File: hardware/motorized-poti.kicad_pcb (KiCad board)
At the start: 2 copper layers, 100 x 18 mm, 18 parts, among them J1 AKL_5_2, P1 CON-SENSOR, P2 MOTORIZED_POTI, U1 M24C64, U2 ZXBM5210, U3 DRILL, U4 DRILL, U5 DRILL, U6 DRILL

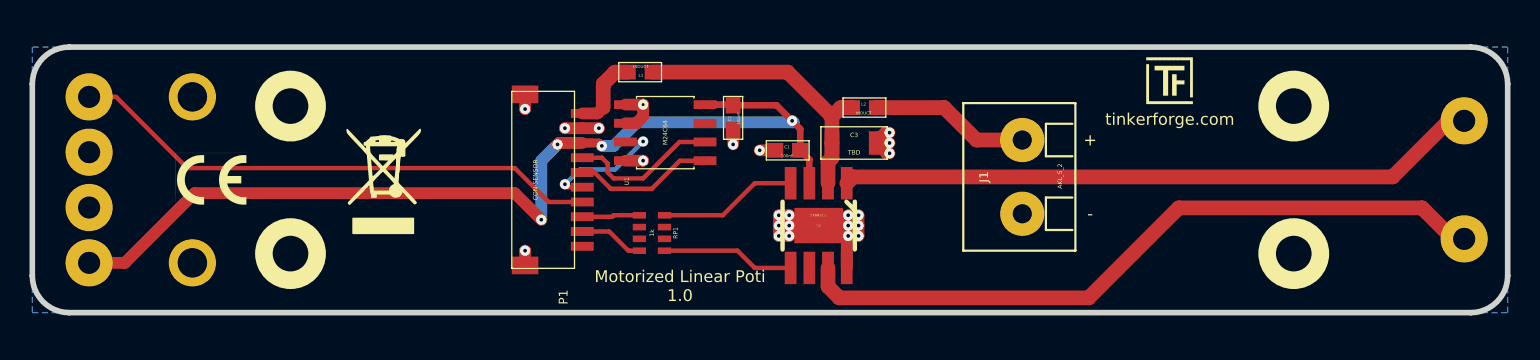
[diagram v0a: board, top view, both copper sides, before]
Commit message: restore proto placement
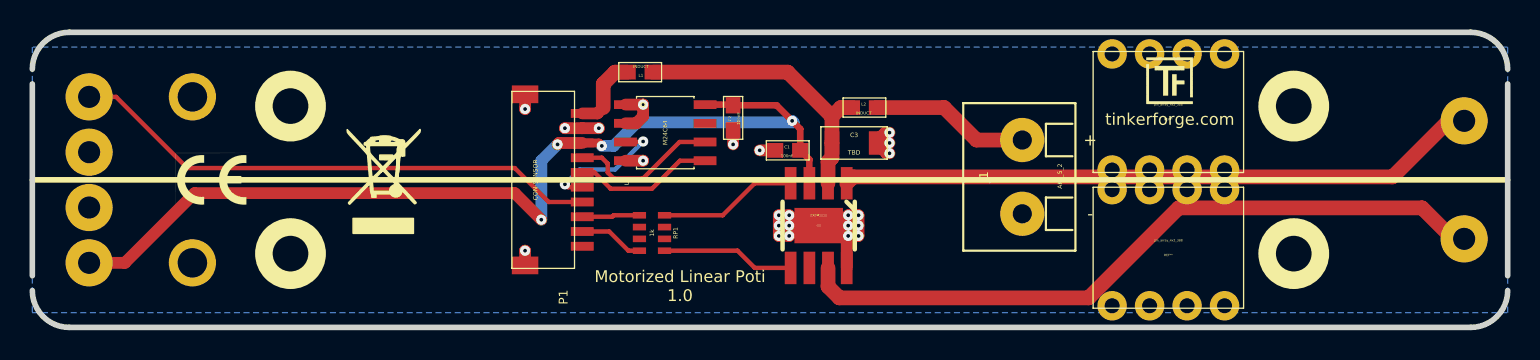
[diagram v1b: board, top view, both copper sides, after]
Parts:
- added REF**: pin_array_4x2_388, kicad-libraries:pin_array_4x2_388, F.Cu at (154.9, 56.4)
- added REF**: pin_array_4x2_388, kicad-libraries:pin_array_4x2_388, F.Cu at (154.9, 47.2)
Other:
- board size 100 x 18 mm -> 100 x 20 mm
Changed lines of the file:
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@@
     (area 71.175139 42.445139 282.895869 162.490743)
     (thickness 1.6002)
-    (drawings 13)
+    (drawings 14)
     (tracks 155)
     (zones 0)
-    (modules 18)
+    (modules 20)
     (nets 16)
   )
@@
       (xy 0.877936 0.493734) (xy 0.931333 0.536222) (xy 0.977806 0.613465) (xy 0.977806 0.613465)) (layer F.SilkS) (width 0.1))
   )
+  (module kicad-libraries:pin_array_4x2_388 (layer Vorderseite)
+    (at 154.9 56.4)
+    (fp_text reference REF** (at 0 0.5) (layer F.SilkS)
+      (effects (font (size 0.15 0.15) (thickness 0.0375)))
+    )
+    (fp_text value pin_array_4x2_388 (at 0 -0.5) (layer F.SilkS)
+      (effects (font (size 0.15 0.15) (thickness 0.0375)))
+    )
+    (fp_line (start -5.1 -4.1) (end 5.1 -4.1) (layer F.SilkS) (width 0.05))
+    (fp_line (start 5.1 -4.1) (end 5.1 4.1) (layer F.SilkS) (width 0.05))
+    (fp_line (start 5.1 4.1) (end -5.1 4.1) (layer F.SilkS) (width 0.05))
+    (fp_line (start -5.1 4.1) (end -5.1 -4.1) (layer F.SilkS) (width 0.05))
+    (pad 1 thru_hole circle (at -3.81 -3.935) (size 2 2) (drill 1.02) (layers *.Cu *.Mask F.SilkS))
+    (pad 3 thru_hole circle (at -1.27 -3.935) (size 2 2) (drill 1.02) (layers *.Cu *.Mask F.SilkS))
+    (pad 5 thru_hole circle (at 1.27 -3.935) (size 2 2) (drill 1.02) (layers *.Cu *.Mask F.SilkS))
+    (pad 7 thru_hole circle (at 3.81 -3.935) (size 2 2) (drill 1.02) (layers *.Cu *.Mask F.SilkS))
+    (pad 2 thru_hole circle (at -3.81 3.935) (size 2 2) (drill 1.02) (layers *.Cu *.Mask F.SilkS))
+    (pad 4 thru_hole circle (at -1.27 3.935) (size 2 2) (drill 1.02) (layers *.Cu *.Mask F.SilkS))
+    (pad 6 thru_hole circle (at 1.27 3.935) (size 2 2) (drill 1.02) (layers *.Cu *.Mask F.SilkS))
+    (pad 8 thru_hole circle (at 3.81 3.935) (size 2 2) (drill 1.02) (layers *.Cu *.Mask F.SilkS))
+  )
+  (module kicad-libraries:pin_array_4x2_388 (layer Vorderseite)
+    (at 154.9 47.2)
+    (fp_text reference REF** (at 0 0.5) (layer F.SilkS)
+      (effects (font (size 0.15 0.15) (thickness 0.0375)))
+    )
+    (fp_text value pin_array_4x2_388 (at 0 -0.5) (layer F.SilkS)
+      (effects (font (size 0.15 0.15) (thickness 0.0375)))
+    )
+    (fp_line (start -5.1 -4.1) (end 5.1 -4.1) (layer F.SilkS) (width 0.05))
+    (fp_line (start 5.1 -4.1) (end 5.1 4.1) (layer F.SilkS) (width 0.05))
+    (fp_line (start 5.1 4.1) (end -5.1 4.1) (layer F.SilkS) (width 0.05))
+    (fp_line (start -5.1 4.1) (end -5.1 -4.1) (layer F.SilkS) (width 0.05))
+    (pad 1 thru_hole circle (at -3.81 -3.935) (size 2 2) (drill 1.02) (layers *.Cu *.Mask F.SilkS))
+    (pad 3 thru_hole circle (at -1.27 -3.935) (size 2 2) (drill 1.02) (layers *.Cu *.Mask F.SilkS))
+    (pad 5 thru_hole circle (at 1.27 -3.935) (size 2 2) (drill 1.02) (layers *.Cu *.Mask F.SilkS))
+    (pad 7 thru_hole circle (at 3.81 -3.935) (size 2 2) (drill 1.02) (layers *.Cu *.Mask F.SilkS))
+    (pad 2 thru_hole circle (at -3.81 3.935) (size 2 2) (drill 1.02) (layers *.Cu *.Mask F.SilkS))
+    (pad 4 thru_hole circle (at -1.27 3.935) (size 2 2) (drill 1.02) (layers *.Cu *.Mask F.SilkS))
+    (pad 6 thru_hole circle (at 1.27 3.935) (size 2 2) (drill 1.02) (layers *.Cu *.Mask F.SilkS))
+    (pad 8 thru_hole circle (at 3.81 3.935) (size 2 2) (drill 1.02) (layers *.Cu *.Mask F.SilkS))
+  )
+  (gr_line (start 177.9 51.8) (end 77.9 51.8) (angle 90) (layer F.SilkS) (width 0.381))
   (gr_text - (at 149.6 54.1) (layer F.SilkS)
     (effects (font (size 0.8001 0.8001) (thickness 0.14986)))
@@
   )
   (gr_line (start 77.9 58.3) (end 77.9 45.3) (angle 90) (layer Edge.Cuts) (width 0.381))
-  (gr_arc (start 80.4 58.3) (end 80.4 60.8) (angle 90) (layer Edge.Cuts) (width 0.381))
-  (gr_line (start 175.4 60.8) (end 80.4 60.8) (angle 90) (layer Edge.Cuts) (width 0.381))
-  (gr_arc (start 80.4 45.3) (end 77.9 45.3) (angle 90) (layer Edge.Cuts) (width 0.381))
-  (gr_line (start 175.4 42.8) (end 80.4 42.8) (angle 90) (layer Edge.Cuts) (width 0.381))
+  (gr_arc (start 80.4 59.3) (end 80.4 61.8) (angle 90) (layer Edge.Cuts) (width 0.381))
+  (gr_line (start 175.4 61.8) (end 80.4 61.8) (angle 90) (layer Edge.Cuts) (width 0.381))
+  (gr_arc (start 80.4 44.3) (end 77.9 44.3) (angle 90) (layer Edge.Cuts) (width 0.381))
+  (gr_line (start 175.4 41.8) (end 80.4 41.8) (angle 90) (layer Edge.Cuts) (width 0.381))
   (gr_line (start 177.9 58.3) (end 177.9 45.3) (angle 90) (layer Edge.Cuts) (width 0.381))
-  (gr_arc (start 175.4 58.3) (end 177.9 58.3) (angle 90) (layer Edge.Cuts) (width 0.381))
-  (gr_arc (start 175.4 45.3) (end 175.4 42.8) (angle 90) (layer Edge.Cuts) (width 0.381))
+  (gr_arc (start 175.4 59.3) (end 177.9 59.3) (angle 90) (layer Edge.Cuts) (width 0.381))
+  (gr_arc (start 175.4 44.3) (end 175.4 41.8) (angle 90) (layer Edge.Cuts) (width 0.381))
   (gr_text "Copyright Tinkerforge GmbH 2015.\nThis documentation describes Open Hardware and is licensed under the\nCERN OHL v. 1.1.\nYou may redistribute and modify this documentation under the terms of the\nCERN OHL v.1.1. (http://ohwr.org/cernohl). This documentation is distributed\nWITHOUT ANY EXPRESS OR IMPLIED WARRANTY, INCLUDING OF\nMERCHANTABILITY, SATISFACTORY QUALITY AND FITNESS FOR A\nPARTICULAR PURPOSE. Please see the CERN OHL v.1.1 for applicable\nconditions" (at 258.8 156.55) (layer Cmts.User)
     (effects (font (size 0.8001 0.8001) (thickness 0.200025) italic))
